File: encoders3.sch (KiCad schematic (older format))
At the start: 45 parts, among them U13 74HCT595, U14 74HC165

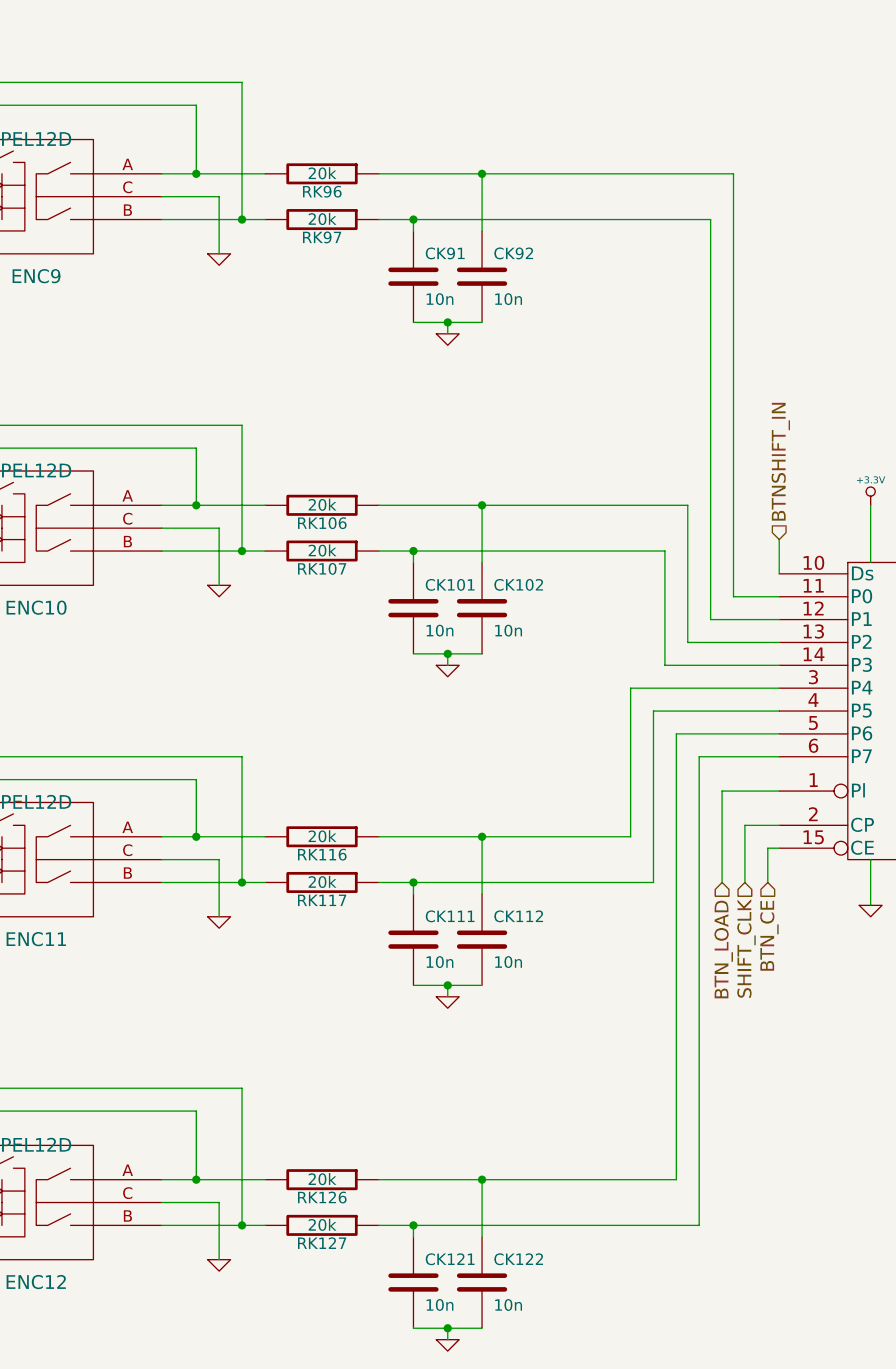
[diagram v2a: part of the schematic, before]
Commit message: Routing.
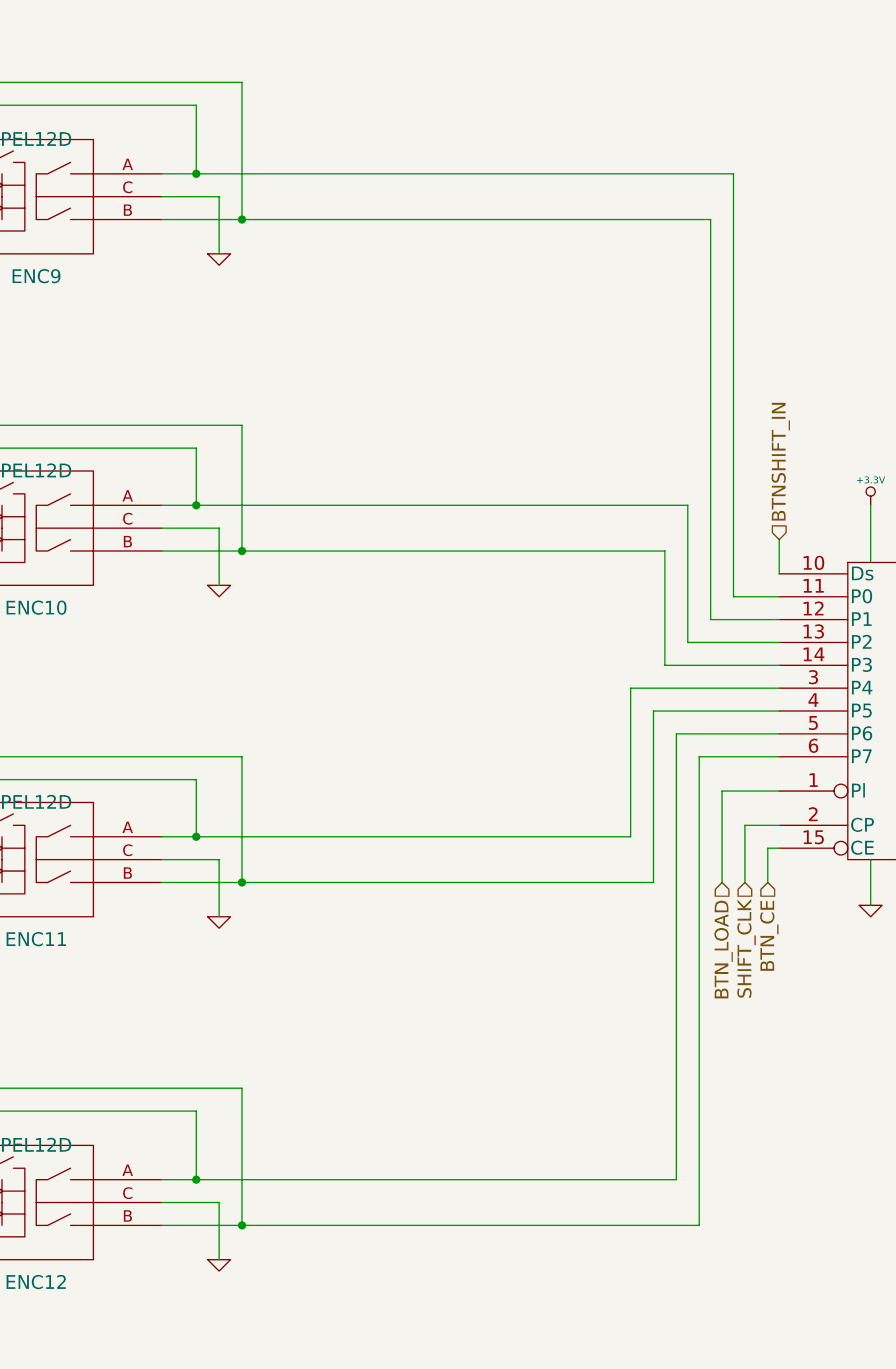
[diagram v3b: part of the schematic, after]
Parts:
- removed CK101, CK102, CK111, CK112, CK121, CK122, CK91, CK92: 10n, symbol C
- removed RK106, RK107, RK116, RK117, RK126, RK127, RK96, RK97: 20k, symbol R
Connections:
- wire segments 173 -> 149

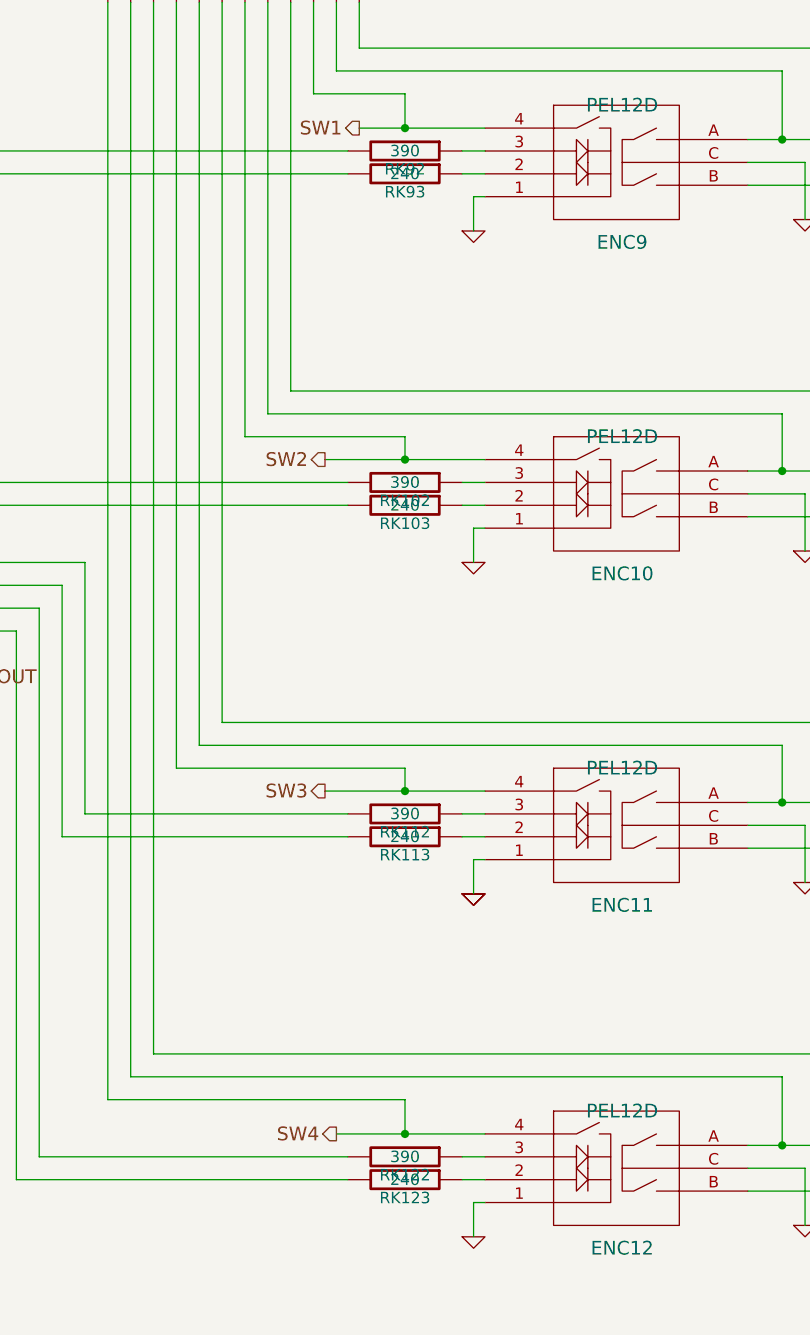
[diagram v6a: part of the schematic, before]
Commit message: Finished board CAD?
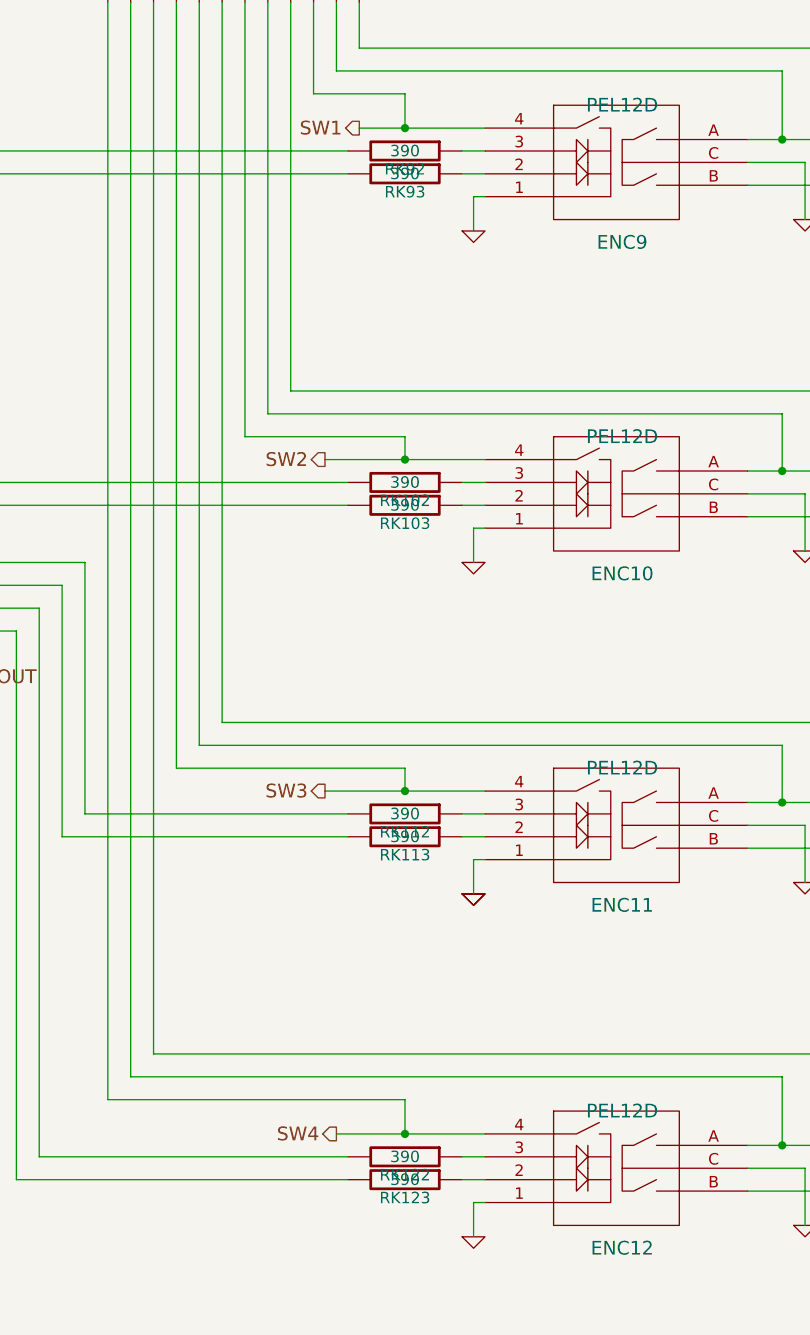
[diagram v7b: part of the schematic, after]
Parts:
- RK103, RK113, RK123, RK93: value 240 -> 390
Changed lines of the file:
@@
-EESchema Schematic File Version 2  date Sat 01 Jun 2013 11:43:44 AM CEST
+EESchema Schematic File Version 2  date Sat 08 Jun 2013 11:15:40 AM CEST
 LIBS:power
 LIBS:device
@@
 Sheet 7 10
 Title ""
-Date "1 jun 2013"
+Date "8 jun 2013"
 Rev ""
 Comp ""
@@
 $EndComp
 $Comp
-L +5V #PWR68
+L +5V #PWR073
 U 1 1 4F905A7D
 P 1050 3200
-F 0 "#PWR68" H 1050 3290 20  0001 C CNN
+F 0 "#PWR073" H 1050 3290 20  0001 C CNN
 F 1 "+5V" H 1050 3290 30  0000 C CNN
 	1    1050 3200
@@
 NXP 74HCT595 will source up to 8mA to each output\nand seems to be 5V/3V compatible.
 $Comp
-L +3.3V #PWR83
+L +3.3V #PWR074
 U 1 1 4F905A7C
 P 10300 5550
-F 0 "#PWR83" H 10300 5510 30  0001 C CNN
+F 0 "#PWR074" H 10300 5510 30  0001 C CNN
 F 1 "+3.3V" H 10300 5660 30  0000 C CNN
 	1    10300 5550
@@
 $EndComp
 $Comp
-L GND #PWR84
+L GND #PWR075
 U 1 1 4F829FCF
 P 10300 6250
-F 0 "#PWR84" H 10300 6250 30  0001 C CNN
+F 0 "#PWR075" H 10300 6250 30  0001 C CNN
 F 1 "GND" H 10300 6180 30  0001 C CNN
 	1    10300 6250
@@
 $EndComp
 $Comp
-L GND #PWR71
+L GND #PWR076
 U 1 1 4F829EA4
 P 1850 7150
-F 0 "#PWR71" H 1850 7150 30  0001 C CNN
+F 0 "#PWR076" H 1850 7150 30  0001 C CNN
 F 1 "GND" H 1850 7080 30  0001 C CNN
 	1    1850 7150
@@
 $EndComp
 $Comp
-L +5V #PWR70
+L +5V #PWR077
 U 1 1 4F92B22F
 P 1850 6500
-F 0 "#PWR70" H 1850 6590 20  0001 C CNN
+F 0 "#PWR077" H 1850 6590 20  0001 C CNN
 F 1 "+5V" H 1850 6590 30  0000 C CNN
 	1    1850 6500
@@
 $EndComp
 $Comp
-L +3.3V #PWR81
+L +3.3V #PWR078
 U 1 1 4F92B268
 P 9450 3500
-F 0 "#PWR81" H 9450 3460 30  0001 C CNN
+F 0 "#PWR078" H 9450 3460 30  0001 C CNN
 F 1 "+3.3V" H 9450 3610 30  0000 C CNN
 	1    9450 3500
@@
 $EndComp
 $Comp
-L GND #PWR82
+L GND #PWR079
 U 1 1 4F92B266
 P 9450 5250
-F 0 "#PWR82" H 9450 5250 30  0001 C CNN
+F 0 "#PWR079" H 9450 5250 30  0001 C CNN
 F 1 "GND" H 9450 5180 30  0001 C CNN
 	1    9450 5250
@@
 Needs to be 5V/3V compatible --> use HCT
 $Comp
-L GND #PWR69
+L GND #PWR080
 U 1 1 4F92B21C
 P 1050 4700
-F 0 "#PWR69" H 1050 4700 30  0001 C CNN
+F 0 "#PWR080" H 1050 4700 30  0001 C CNN
 F 1 "GND" H 1050 4630 30  0001 C CNN
 	1    1050 4700
@@
 $EndComp
 $Comp
-L GND #PWR74
+L GND #PWR081
 U 1 1 4F92B21A
 P 5150 5350
-F 0 "#PWR74" H 5150 5350 30  0001 C CNN
+F 0 "#PWR081" H 5150 5350 30  0001 C CNN
 F 1 "GND" H 5150 5280 30  0001 C CNN
 	1    5150 5350
@@
 $EndComp
 $Comp
-L GND #PWR72
+L GND #PWR082
 U 1 1 4F92B262
 P 5150 2450
-F 0 "#PWR72" H 5150 2450 30  0001 C CNN
+F 0 "#PWR082" H 5150 2450 30  0001 C CNN
 F 1 "GND" H 5150 2380 30  0001 C CNN
 	1    5150 2450
@@
 P 4850 2200
 F 0 "RK93" V 4930 2200 50  0000 C CNN
-F 1 "240" V 4850 2200 50  0000 C CNN
+F 1 "390" V 4850 2200 50  0000 C CNN
 	1    4850 2200
 	0    1    1    0
 $EndComp
 $Comp
-L GND #PWR77
+L GND #PWR083
 U 1 1 4F905A62
 P 6600 2400
-F 0 "#PWR77" H 6600 2400 30  0001 C CNN
+F 0 "#PWR083" H 6600 2400 30  0001 C CNN
 F 1 "GND" H 6600 2330 30  0001 C CNN
 	1    6600 2400
@@
 $EndComp
 $Comp
-L GND #PWR78
+L GND #PWR084
 U 1 1 4F92B24F
 P 6600 3850
-F 0 "#PWR78" H 6600 3850 30  0001 C CNN
+F 0 "#PWR084" H 6600 3850 30  0001 C CNN
 F 1 "GND" H 6600 3780 30  0001 C CNN
 	1    6600 3850
@@
 P 4850 3650
 F 0 "RK103" V 4930 3650 50  0000 C CNN
-F 1 "240" V 4850 3650 50  0000 C CNN
+F 1 "390" V 4850 3650 50  0000 C CNN
 	1    4850 3650
 	0    1    1    0
@@
 $EndComp
 $Comp
-L GND #PWR73
+L GND #PWR085
 U 1 1 4F905A54
 P 5150 3900
-F 0 "#PWR73" H 5150 3900 30  0001 C CNN
+F 0 "#PWR085" H 5150 3900 30  0001 C CNN
 F 1 "GND" H 5150 3830 30  0001 C CNN
 	1    5150 3900
@@
 $EndComp
 $Comp
-L GND #PWR75
+L GND #PWR086
 U 1 1 4F92B246
 P 5150 5350
-F 0 "#PWR75" H 5150 5350 30  0001 C CNN
+F 0 "#PWR086" H 5150 5350 30  0001 C CNN
 F 1 "GND" H 5150 5280 30  0001 C CNN
 	1    5150 5350
@@
 P 4850 5100
 F 0 "RK113" V 4930 5100 50  0000 C CNN
-F 1 "240" V 4850 5100 50  0000 C CNN
+F 1 "390" V 4850 5100 50  0000 C CNN
 	1    4850 5100
 	0    1    1    0
 $EndComp
 $Comp
-L GND #PWR79
+L GND #PWR087
 U 1 1 4F92B208
 P 6600 5300
-F 0 "#PWR79" H 6600 5300 30  0001 C CNN
+F 0 "#PWR087" H 6600 5300 30  0001 C CNN
 F 1 "GND" H 6600 5230 30  0001 C CNN
 	1    6600 5300
@@
 $EndComp
 $Comp
-L GND #PWR80
+L GND #PWR088
 U 1 1 4F905A43
 P 6600 6800
-F 0 "#PWR80" H 6600 6800 30  0001 C CNN
+F 0 "#PWR088" H 6600 6800 30  0001 C CNN
 F 1 "GND" H 6600 6730 30  0001 C CNN
 	1    6600 6800
@@
 P 4850 6600
 F 0 "RK123" V 4930 6600 50  0000 C CNN
-F 1 "240" V 4850 6600 50  0000 C CNN
+F 1 "390" V 4850 6600 50  0000 C CNN
 	1    4850 6600
 	0    1    1    0
@@
 $EndComp
 $Comp
-L GND #PWR76
+L GND #PWR089
 U 1 1 4F92B1F9
 P 5150 6850
-F 0 "#PWR76" H 5150 6850 30  0001 C CNN
+F 0 "#PWR089" H 5150 6850 30  0001 C CNN
 F 1 "GND" H 5150 6780 30  0001 C CNN
 	1    5150 6850
